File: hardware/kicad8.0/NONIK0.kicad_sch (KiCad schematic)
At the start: 18 parts, among them J1 AVR-UPDI-6, J2 Qwiic/Stemma QT, J3 Test Pads, SW1 SW_SPST, SW2 SW_Push, SW3 SW_Push, U1 HCMS-291X, U2 ATtiny1604-SS

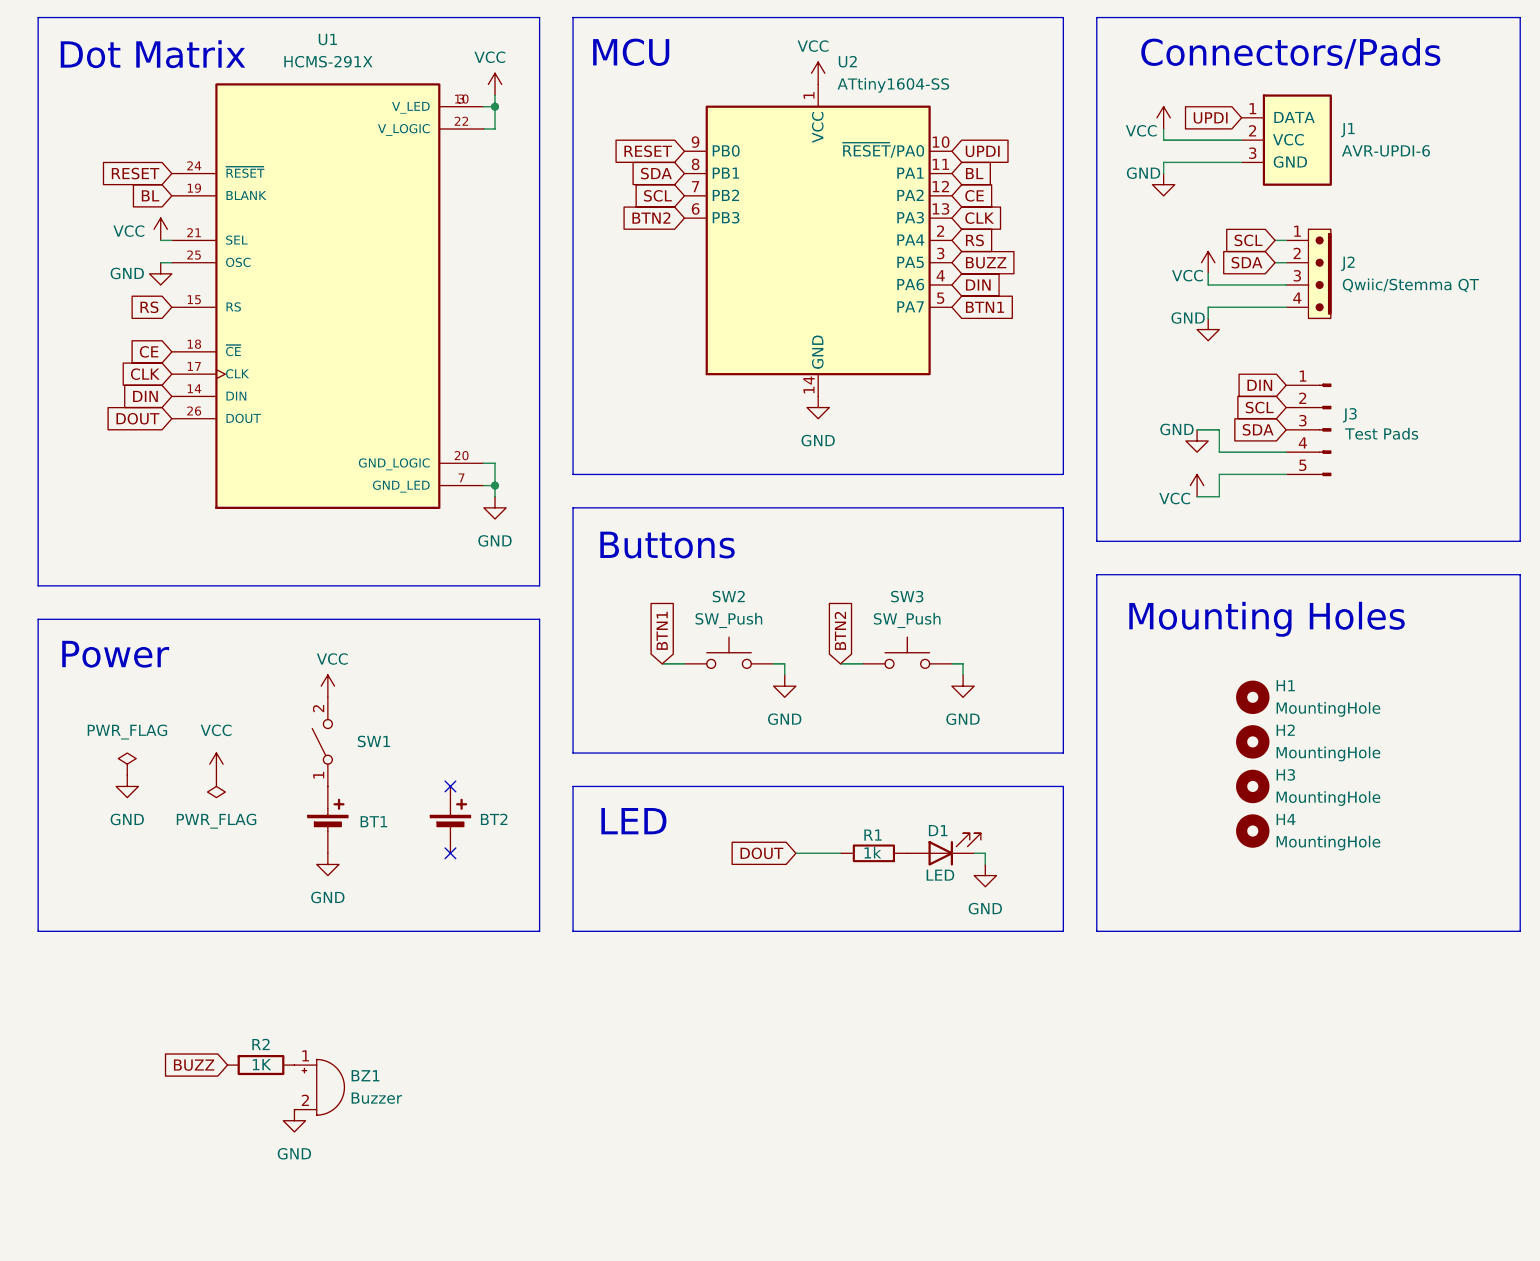
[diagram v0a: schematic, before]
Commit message: adding power reg and piezo
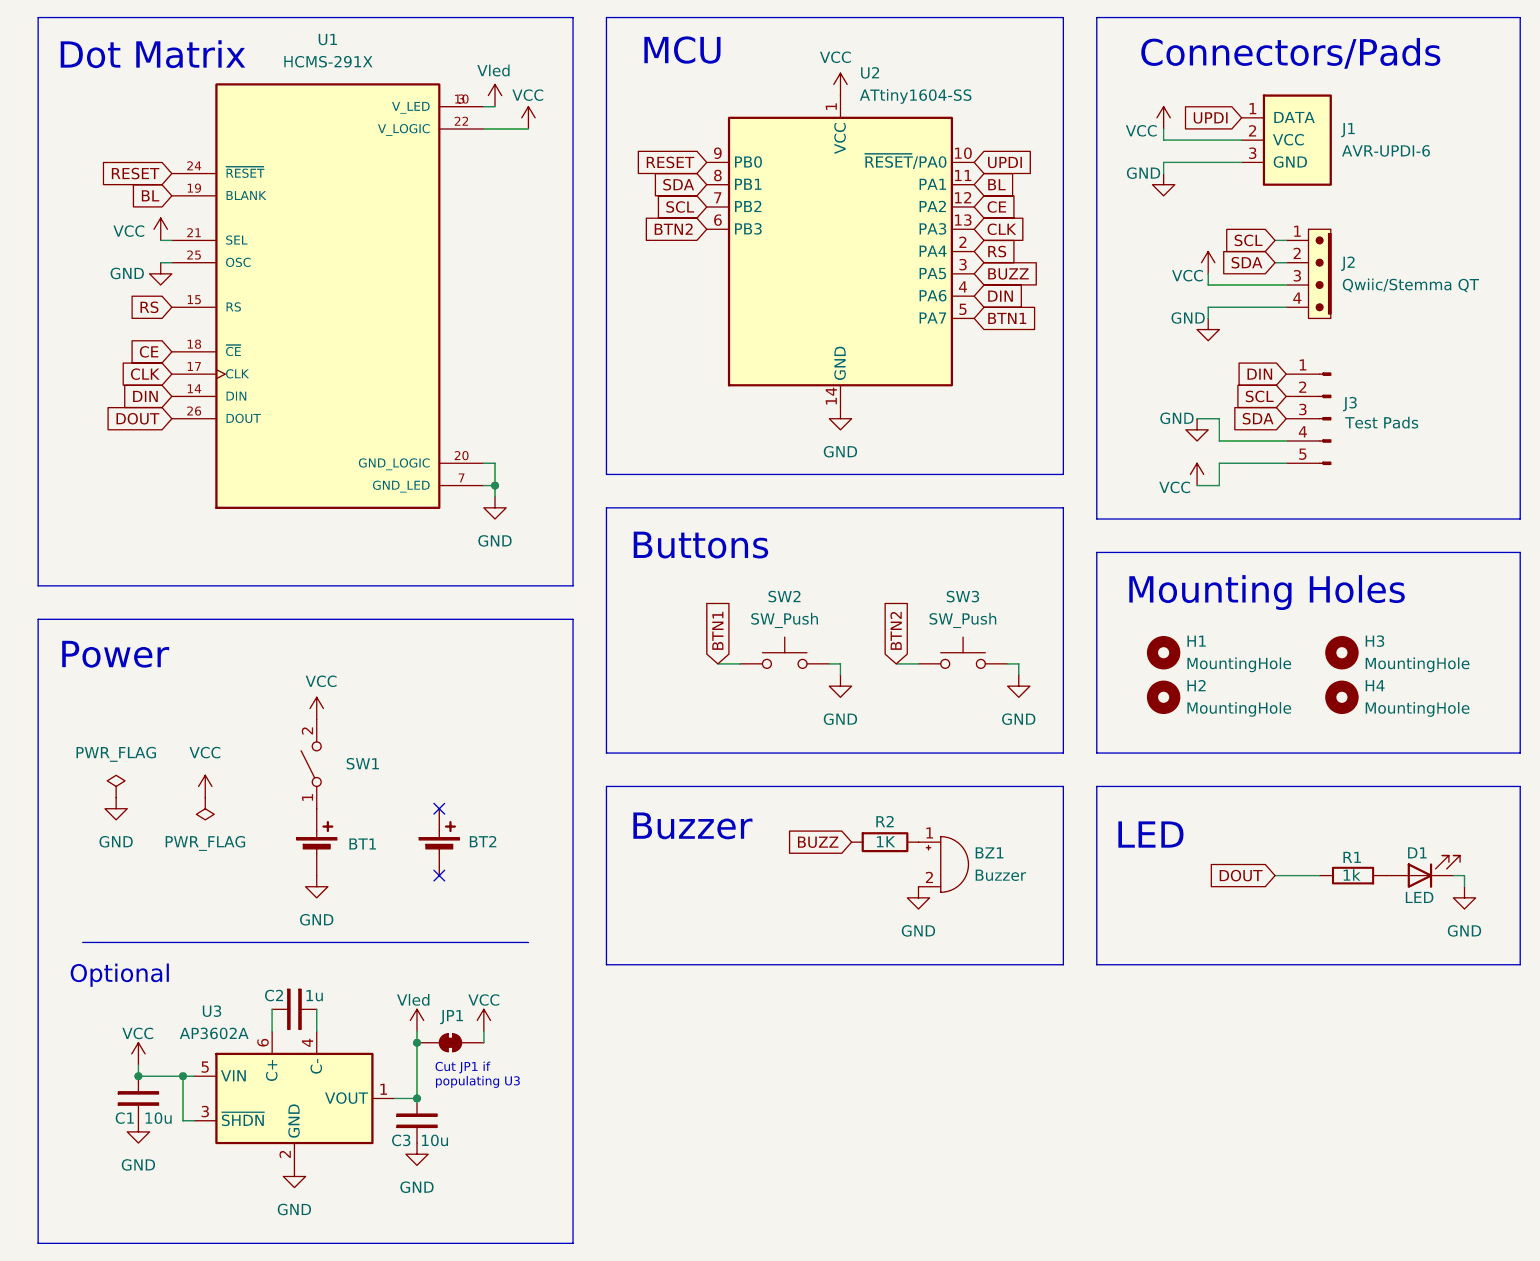
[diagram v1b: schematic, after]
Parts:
- added C1, C3: 10u, NONIK0:C_0603_1608Metric, symbol PCM_SL_Devices:Capacitor_NP
- added C2: 1u, NONIK0:C_0603_1608Metric, symbol PCM_SL_Devices:Capacitor_NP
- added JP1: SolderJumper_2_Bridged, Jumper:SolderJumper-3_P1.3mm_Bridged2Bar12_RoundedPad1.0x1.5mm, symbol Jumper:SolderJumper_2_Bridged
- added U3: AP3602A, NONIK0:SOT-23-6, symbol NONIK0:AP3602A
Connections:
- net GND: now also C1.1, C3.1, U3.2 (GND)
- net VCC: now also C1.2, JP1.2 (B), U3.3 (~{SHDN}), U3.5 (VIN); no longer U1.10 (V_LED), U1.3 (V_LED)
- new net: C2.1, U3.6 (C+)
- new net: C2.2, U3.4 (C-)
- new net Vled: C3.2, JP1.1 (A), U1.10 (V_LED), U1.3 (V_LED), U3.1 (VOUT)
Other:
- note added: "Buzzer"
- note added: "Cut JP1 if populating U3"
- note added: "Optional"
- moved on the sheet: BT1, BT2, BZ1, D1, H1, H2, H3, H4, J3, R1, R2, SW1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

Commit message: pcb done, pending review
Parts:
- JP1: footprint Jumper:SolderJumper-3_P1.3mm_Bridged2Bar12_RoundedPad1.0x1.5mm -> NONIK0:SolderJumper-2_P1.3mm_Bridged_RoundedPad1.0x1.5mm
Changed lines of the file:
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@@
 			)
 		)
-		(property "Footprint" "Jumper:SolderJumper-3_P1.3mm_Bridged2Bar12_RoundedPad1.0x1.5mm"
+		(property "Footprint" "NONIK0:SolderJumper-2_P1.3mm_Bridged_RoundedPad1.0x1.5mm"
 			(at 62.23 132.08 0)
 			(effects

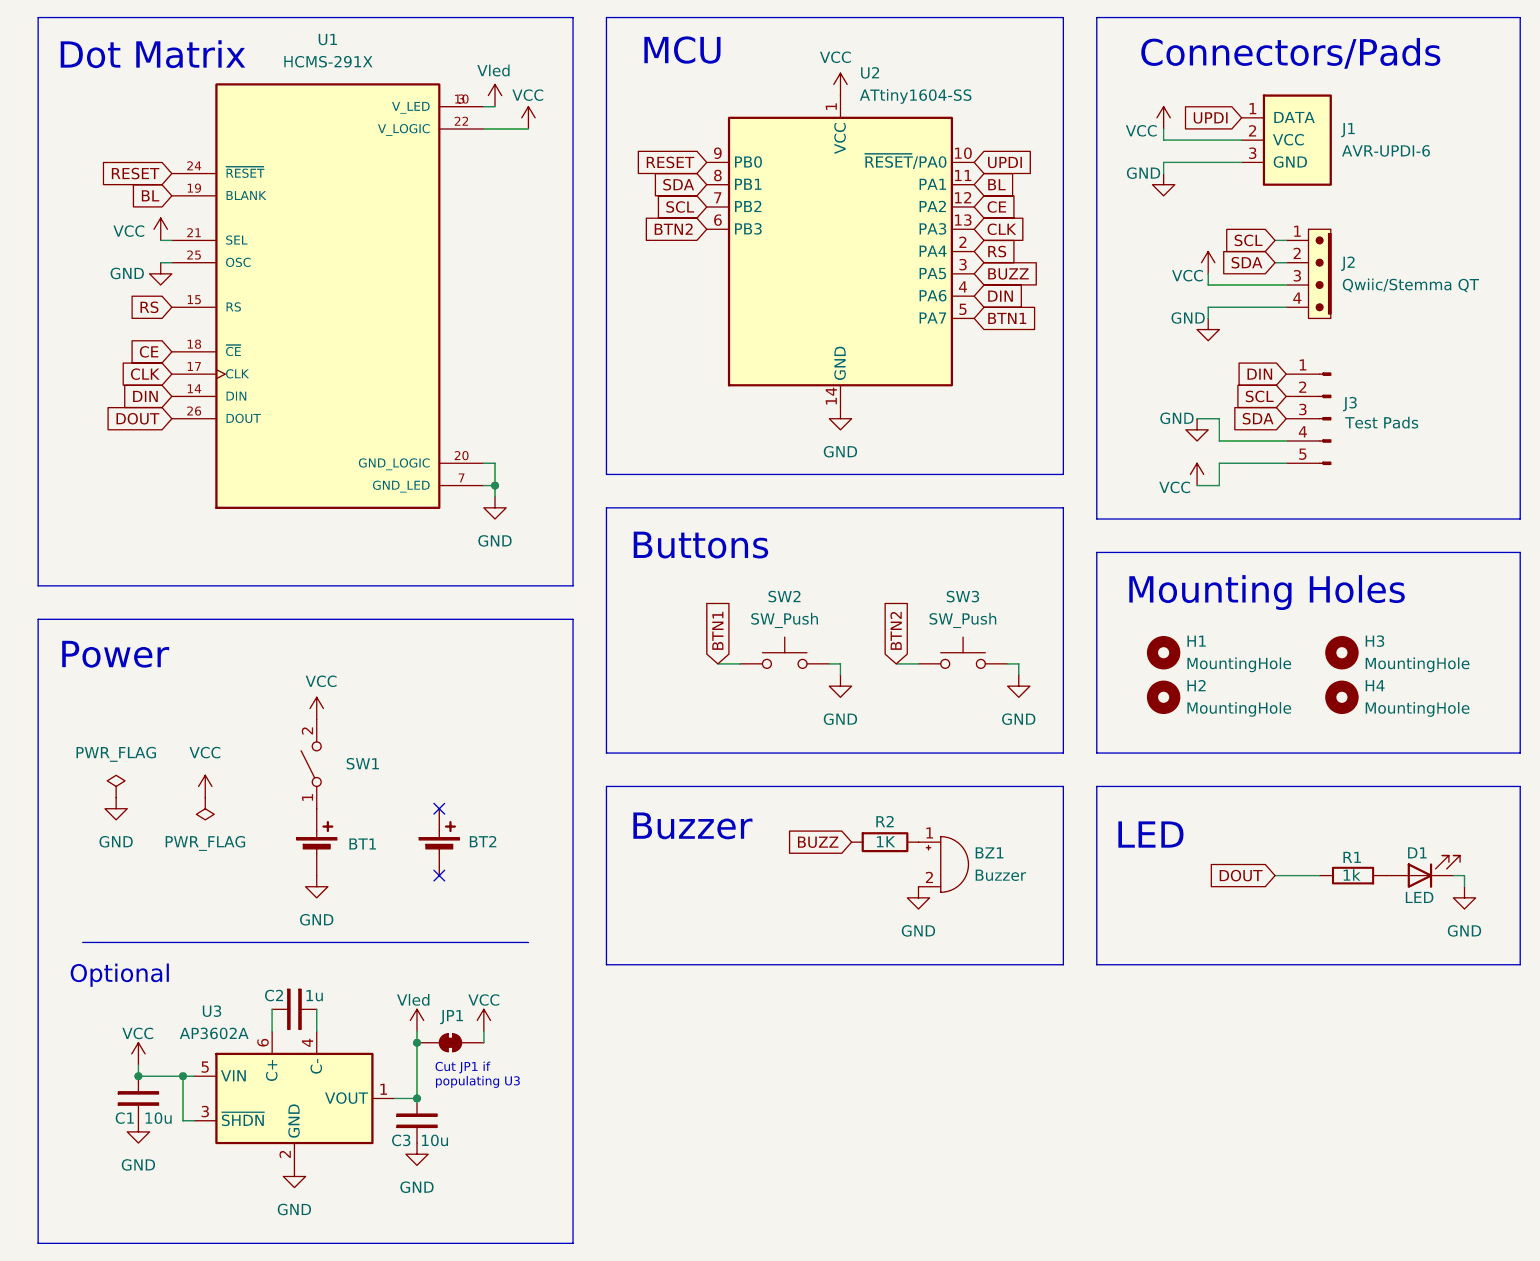
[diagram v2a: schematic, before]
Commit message: fit and finish things
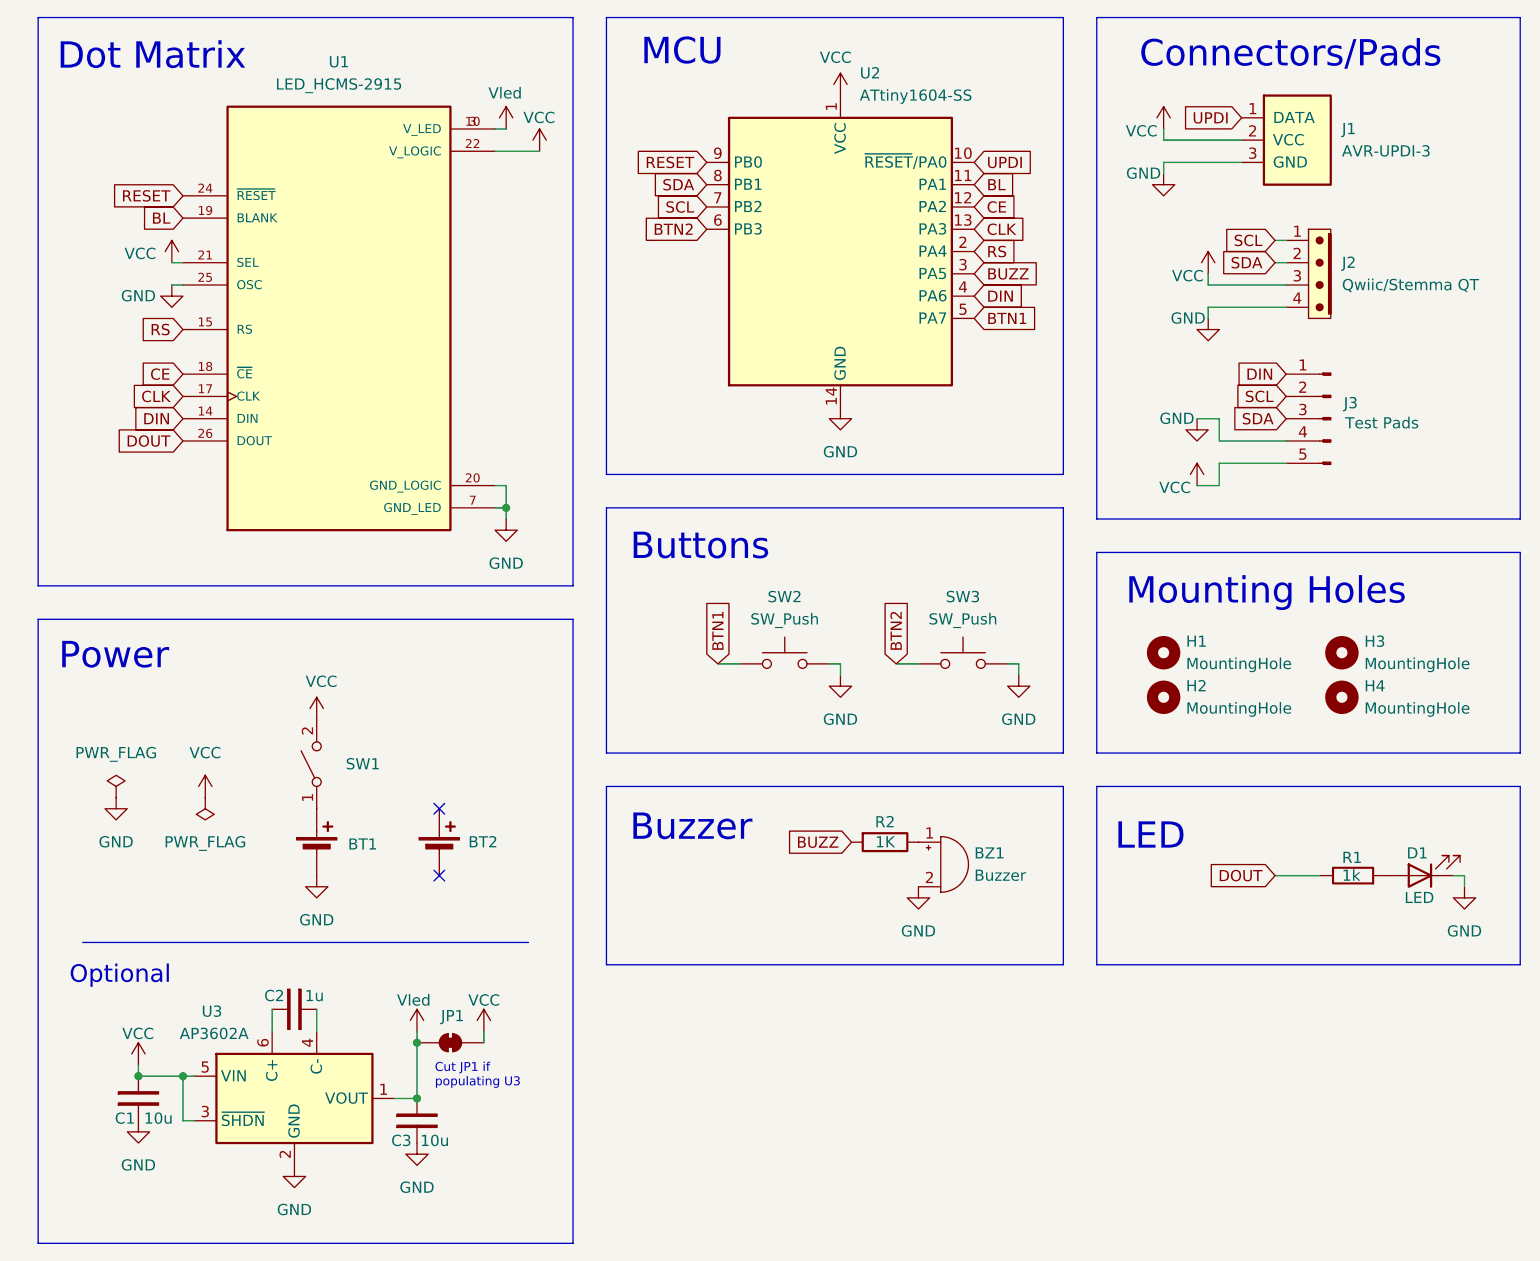
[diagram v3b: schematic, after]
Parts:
- J1: value AVR-UPDI-6 -> AVR-UPDI-3
- U1: value HCMS-291X -> LED_HCMS-2915
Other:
- moved on the sheet: U1
